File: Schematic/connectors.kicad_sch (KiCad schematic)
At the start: 32 parts, among them J10 PIN2216, J11 PIN2216, J12 PIN2216, J2 PIN2216, J3 PIN2216, J4 PIN2216, J5 PIN2216, J6 PIN2216, J7 PIN2216, J8 PIN2216, J9 PIN2216, U14 HDGC1002WR-S-4P, U15 HDGC1002WR-S-4P, U16 HDGC1002WR-S-4P, U17 HDGC1002WR-S-4P, U19 HDGC1002WR-S-4P, U21 HDGC1002WR-S-8P, U22 HDGC1002WR-S-8P, U23 HDGC1002WR-S-6P, U24 HDGC1002WR-S-4P

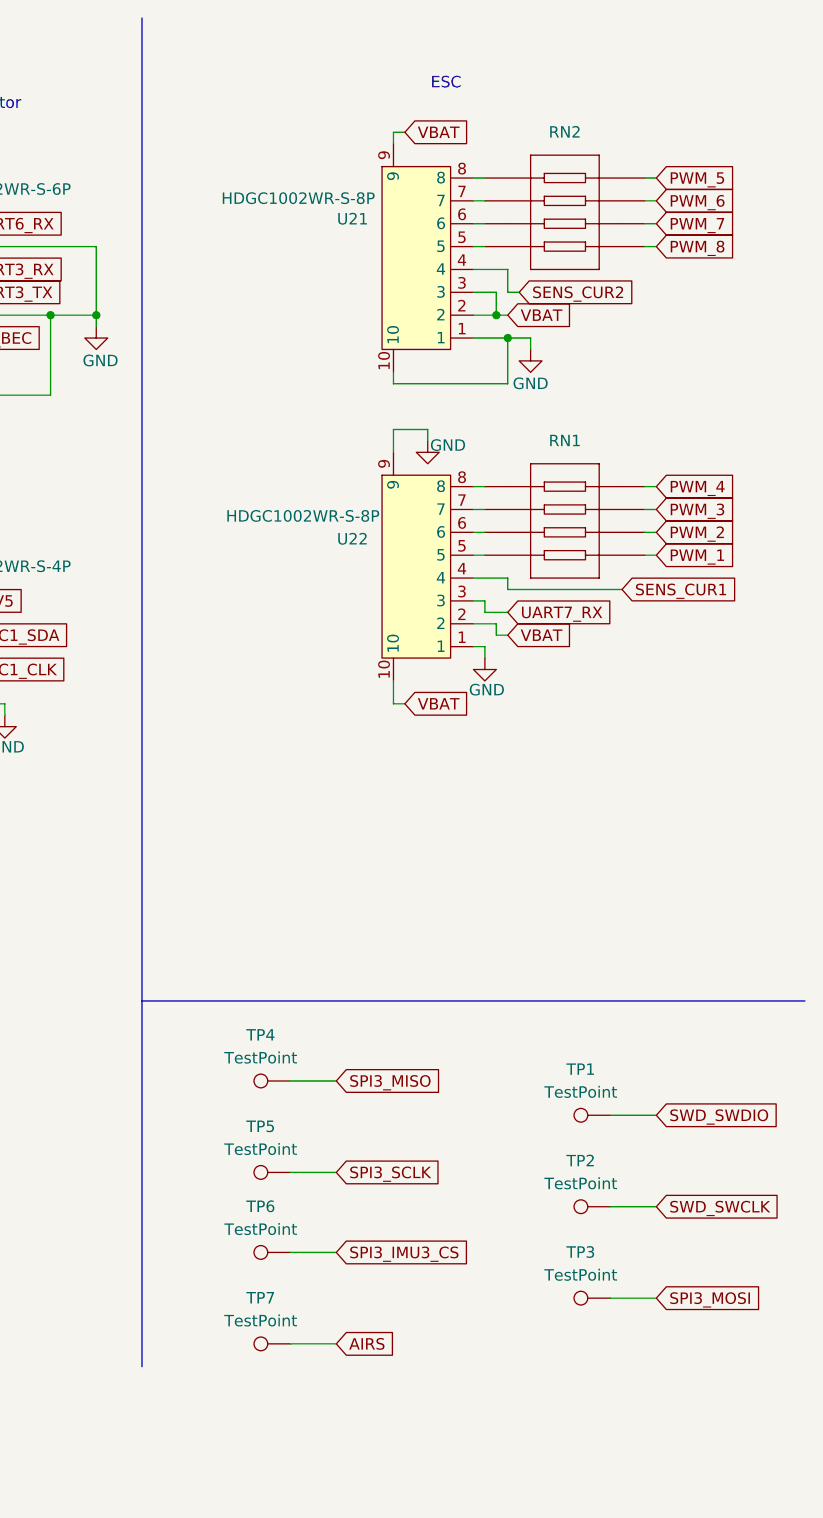
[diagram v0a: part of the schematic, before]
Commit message: zdd :minor improvements
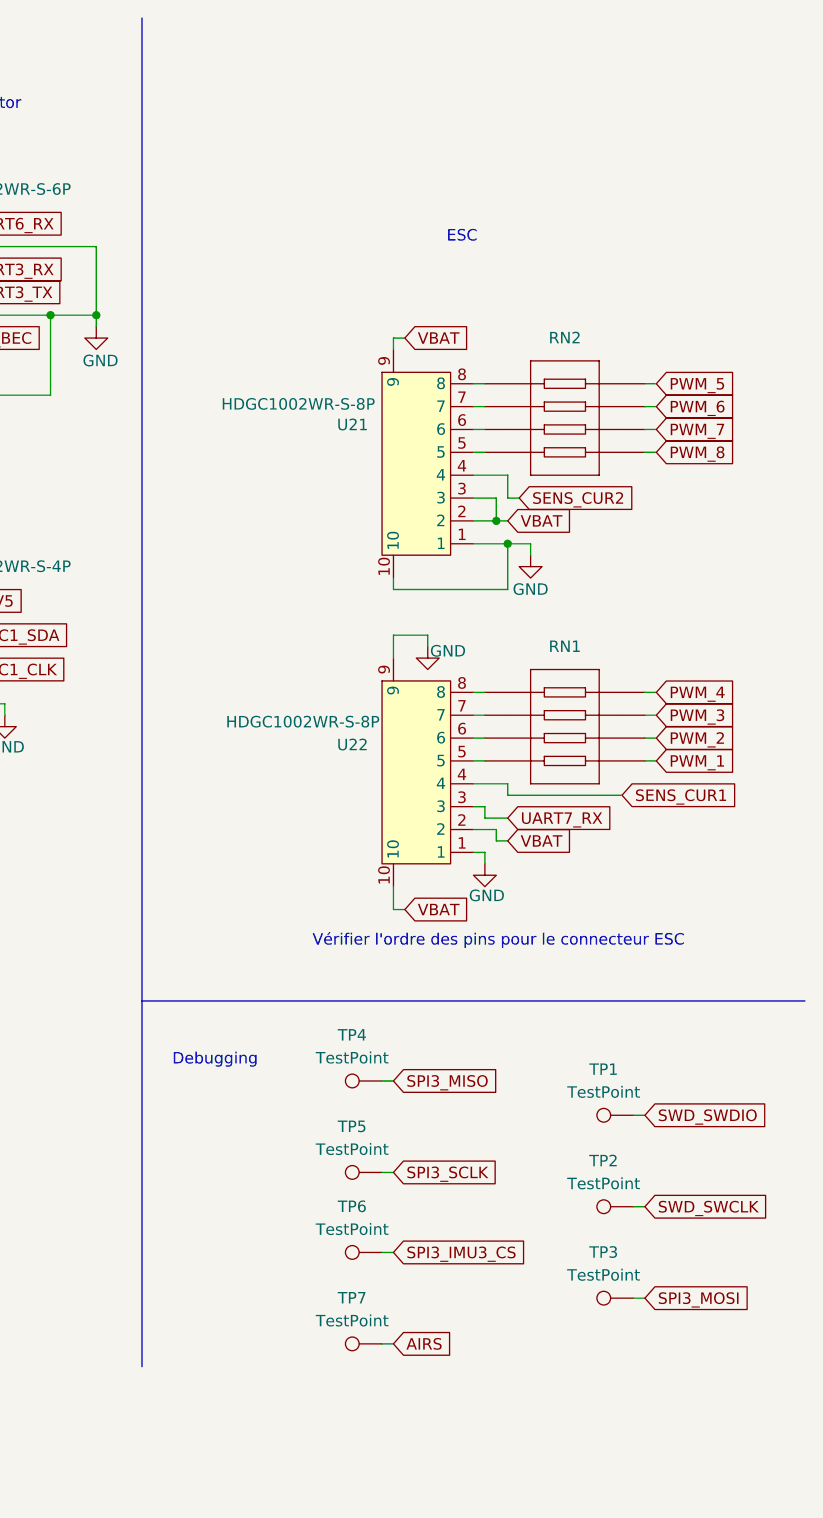
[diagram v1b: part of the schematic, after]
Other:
- note added: "Debugging"
- note added: "Vérifier l'ordre des pins pour le connecteur ESC"
- moved on the sheet: RN1, RN2, TP1, TP2, TP3, TP4, TP5, TP6, TP7, U21, U22
